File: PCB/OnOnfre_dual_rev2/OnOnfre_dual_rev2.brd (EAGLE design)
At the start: 42.4 x 43 mm, 11 parts, among them K1 OMRON-G3MB-202P-SSR2, Q1 S8050

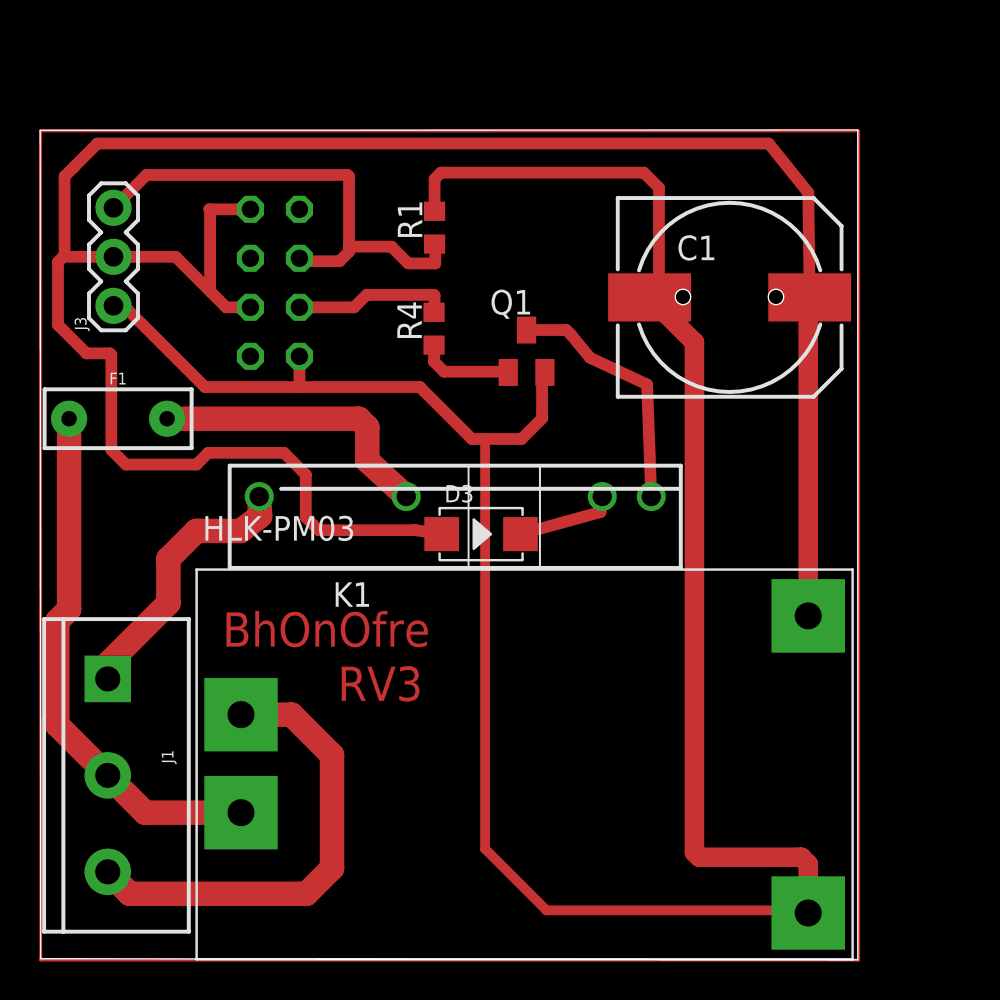
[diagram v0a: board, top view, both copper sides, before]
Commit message: Organização do repositorio
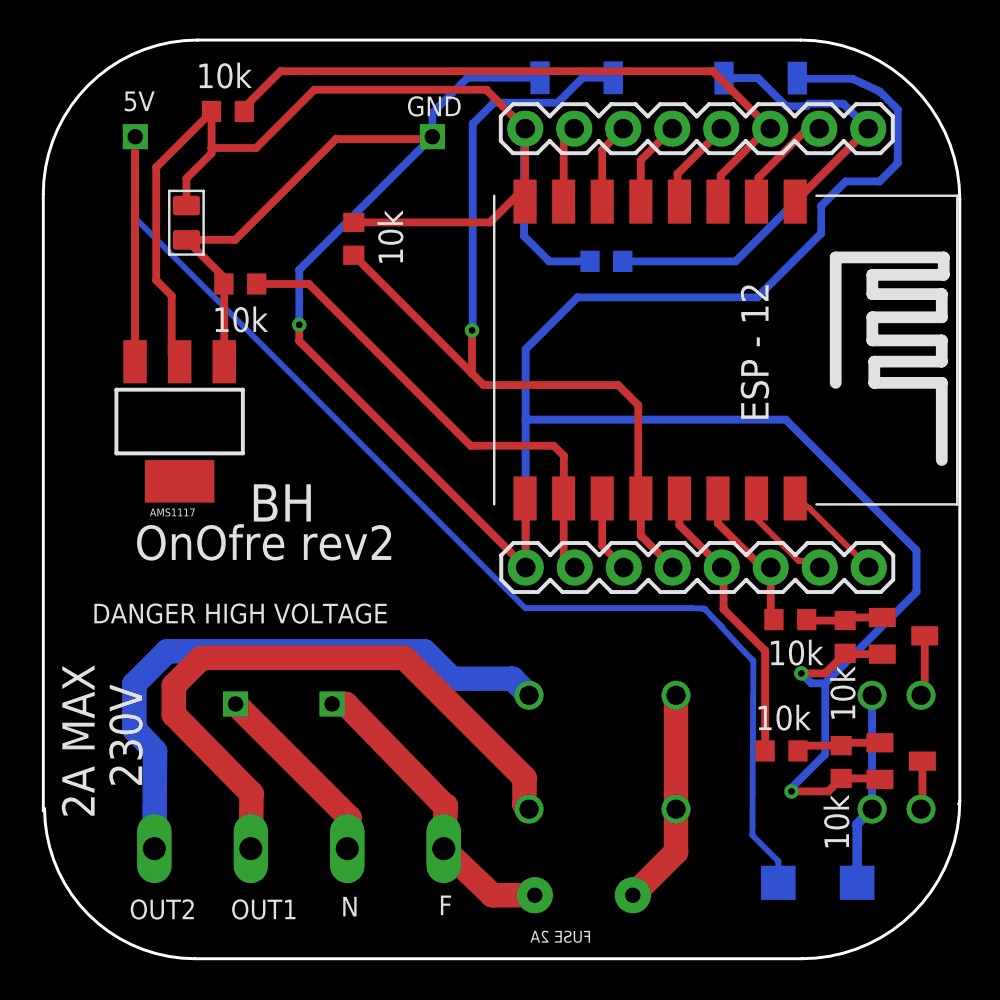
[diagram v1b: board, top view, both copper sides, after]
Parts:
- removed C1: 1000uf, adafruit:140CLH-1010
- removed J1: (no value), SparkFun-Connectors:SCREWTERMINAL-5MM-3
- removed J3: (no value), SparkFun-Connectors:1X03
- removed U$3: ESP8266-01, captain-slow:ESP8266-01
- added AMS1117: LM1117, SparkFun-IC-Power:SOT223
- added C4: 100nf, Seeed-Capacitor:C0805
- added FLASH, RESET: B3U-1000P-2P-SMD, Seeed-Switch:SW2-2.6-3.0X2.5X1.2+0.4MM
- added J6, J7: 8p, SparkFun-Connectors:1X08
- added JY3: S8050, semicon-smd-ipc:SOT23
- added K2: OMRON-G3MB-202P-SSR2, Omron G3MB 202p SSR:OMRON-G3MB-202P-SSR
- added R10, R11, R2, R3, R8, R9: 10k, resistor:R0603
- added U2: esp12, esp8266modules:ESP12-SMD
- added X2: PLUG, con-wago-500:W237-4
- R1, R4: value 47k -> 10k
- U$2: value HLK-PM03 -> HKLPM01; device PowerSocket:HLK-PM03 -> HKLPM01:HKLPM01
- moved F1 34.5 mm to (28.2, 3.29), flipped to the bottom, turned to 180 degrees
- moved Q1 28.8 mm to (44.6, 10.2), turned to 270 degrees
- moved R4 28.3 mm to (38.4, 10.8), turned to 0 degrees
- moved R1 27.4 mm to (38.9, 17.6), turned to 0 degrees
- moved D3 25.1 mm to (40.3, 3.94), flipped to the bottom, turned to 180 degrees
- moved K1 21.4 mm to (38.0, 7.75), flipped to the bottom, turned to 180 degrees
- moved U$2 20.5 mm to (12.6, 27.9), flipped to the bottom, turned to 90 degrees
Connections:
- removed net CH1: R4.2, U$3.GPIO2
- removed net N$4: F1.P$1, J1.2, U$2.AC2
- removed net N$5: J1.3, U$2.AC1
- removed net N$8: D3.2, K1.3
- removed net TOUCH: J3.3, R1.1, U$3.GPIO0
- new net 3V3: AMS1117.2, C4.1, J7.1, R10.2, R8.2, R9.2, U2.VCC
- new net ADC: J7.7, U2.ADC
- new net CH_PD: J7.6, R9.1, U2.CH_PD
- new net FASE_IN: U$2.P$2, X2.2
- new net GPIO0: FLASH.1, J6.4, R8.1, U2.GPIO0
- new net GPIO02: J6.3, U2.GPIO2
- new net GPIO04: J6.6, R1.1, U2.GPIO4
- new net GPIO05: J6.5, R4.1, U2.GPIO5
- new net GPIO12: J7.3, U2.GPIO12
- new net GPIO13: J7.2, U2.GPIO13
- new net GPIO14: J7.4, U2.GPIO14
- new net GPIO15: J6.2, R11.1, U2.GPIO15
- new net GPIO16: J7.5, U2.GPIO16
- new net N$13: JY3.1, R1.2, R2.2
- new net NEUTRAL_IN: F1.P$1, U$2.P$1, X2.1
- new net NEUTRAL_IN_FUSED: F1.P$2, K1.2, K2.2
- new net NEUTRAL_ONE_OUT: K1.1, X2.3
- new net NEUTRAL_TWO_OUT: K2.1, X2.4
- new net RESET: J7.8, R10.1, RESET.1, U2.RESET
- new net RX: J6.7, U2.RXD0
- new net TX: J6.8, U2.TXD0
- net GND: now also AMS1117.1, C4.2, FLASH.2, J6.1, JY3.2, R11.2, R2.1, R3.1, RESET.2, U$2.P$3, U2.GND; no longer C1.-, J3.1, R1.2, U$2.-VO, U$3.GND
- net N$2: now also D3.2, K1.3, K2.3; no longer J1.1, K1.1
- net N$7: now also Q1.1, R3.2, R4.2; no longer F1.P$2, K1.2
- net N$9: now also JY3.3, K2.4; no longer Q1.1, R4.1
- net VCC: now also AMS1117.3, U$2.P$4; no longer C1.+, J3.2, U$2.+VO, U$3.3V3, U$3.CH_PD
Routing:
- net N$3: track 170.6 -> 0.00 mm
- net 3V3: track 0.00 -> 62.3 mm
- net GPIO0: track 0.00 -> 49.3 mm, vias 0 -> 1
- net VCC: track 116.9 -> 69.5 mm
- net CH_PD: track 0.00 -> 34.4 mm
- net NEUTRAL_ONE_OUT: track 0.00 -> 33.2 mm
- net NEUTRAL_TWO_OUT: track 0.00 -> 31.1 mm
- net GND: track 127.0 -> 156.7 mm, vias 0 -> 3
- net RESET: track 0.00 -> 29.6 mm
- net N$4: track 27.9 -> 0.00 mm
- net GPIO15: track 0.00 -> 25.6 mm
- net TOUCH: track 25.5 -> 0.00 mm
- net N$5: track 24.1 -> 0.00 mm
- net NEUTRAL_IN: track 0.00 -> 16.0 mm
- net GPIO05: track 0.00 -> 15.0 mm
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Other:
- board size 42.4 x 43 mm -> 47.5 x 47.6 mm
- board text added: "00"
- board text added: "02"
- board text added: "04"
- board text added: "05"
- board text added: "12"
- board text added: "13"
- board text added: "14"
- board text added: "15"
- board text added: "16"
- board text added: "230V"
- board text added: "2A MAX"
- board text added: "3V3"
- board text added: "5V"
- board text added: "ADC"
- board text added: "BH"
- board text added: "DANGER HIGH VOLTAGE"
- board text added: "EN"
- board text added: "F"
- board text added: "FUSE 2A"
- board text added: "GND"
- board text added: "N"
- board text added: "OUT1"
- board text added: "OUT2"
- board text added: "OnOfre rev2"
- board text added: "RST"
- board text added: "RX"
- board text added: "TX"
- board text added: "www.movimentomaker.pt"
- board text removed: "BhOnOfre"
- board text removed: "RV3"
